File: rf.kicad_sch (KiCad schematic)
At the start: 4 parts, among them J2 ANT_A, J3 ANT_B, U2 SA868

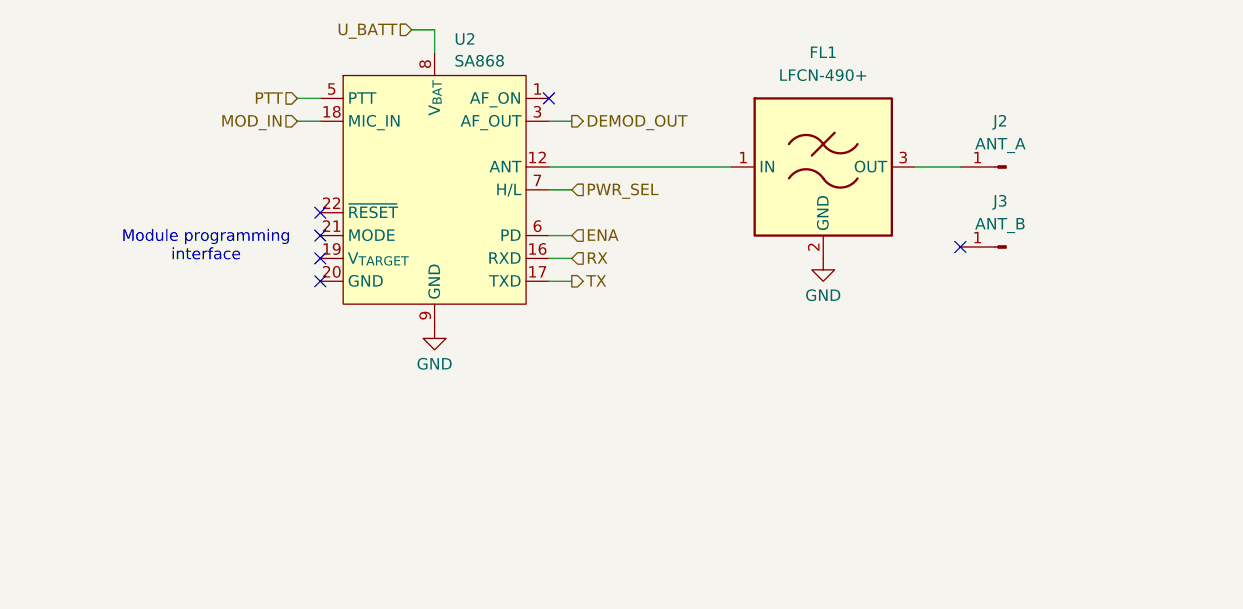
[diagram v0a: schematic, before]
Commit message: audio part
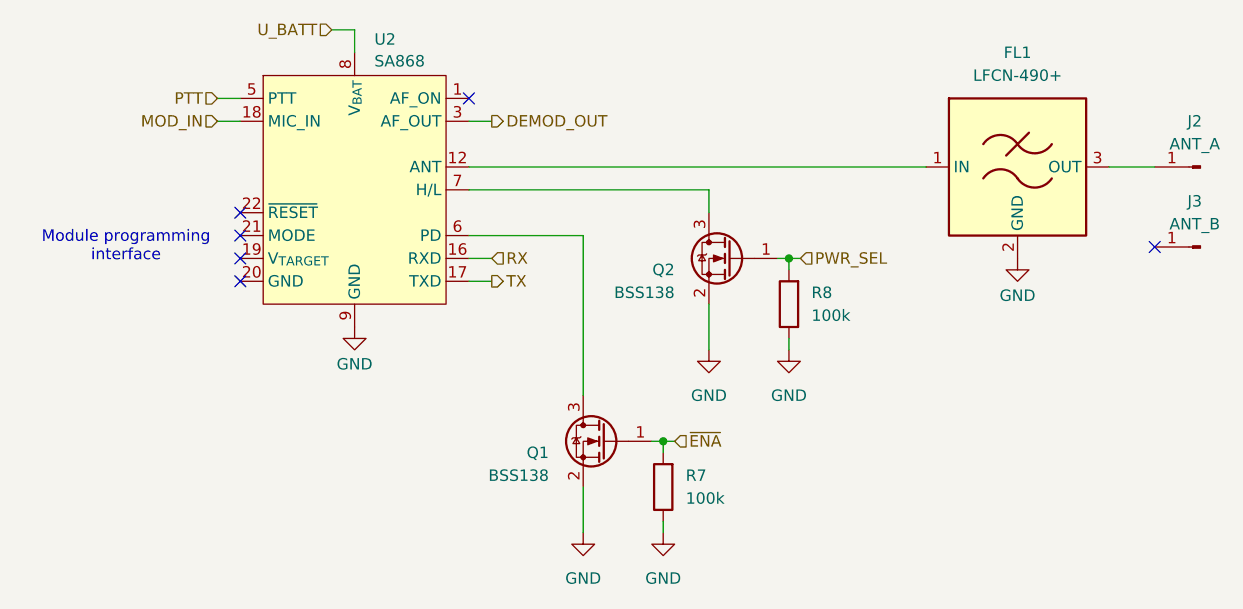
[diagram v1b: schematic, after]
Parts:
- added Q1, Q2: BSS138, Package_TO_SOT_SMD:SOT-23, symbol Transistor_FET:BSS138
- added R7, R8: 100k, Inductor_SMD:L_0805_2012Metric, symbol Device:R
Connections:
- net GND: now also Q1.2 (S), Q2.2 (S), R7.1, R8.1
- net PWR_SEL: now also Q2.1 (G), R8.2; no longer U2.7 (H/L)
- net ENA: no longer names the net of U2.6 (PD)
- net ENA: now also Q1.3 (D)
- new net: Q2.3 (D), U2.7 (H/L)
- new net ~{ENA}: Q1.1 (G), R7.2
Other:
- moved on the sheet: FL1, J2, J3, U2
